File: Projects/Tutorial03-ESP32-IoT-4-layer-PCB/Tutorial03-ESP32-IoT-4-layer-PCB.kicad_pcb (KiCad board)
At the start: 4 copper layers, 149.8 x 55.8 mm, 88 parts, among them J1 SS-52400-002, J2 B2B-PH-SM4-TB, J3 GSD090012SEU, J4 Conn_01x04_Pin, J5 Conn_01x05_Pin, Q1 TEMT6000X01, Q2 BC817, Q3 BC817, U1 MCP73871, U2 MAX4466EXK, U3 ESP32-C3-WROOM-02-H4, U4 CP2102N-Axx-xQFN20, U5 USBLC6-2SC6, U6 W25Q32JVSSIQ, U7 BME280

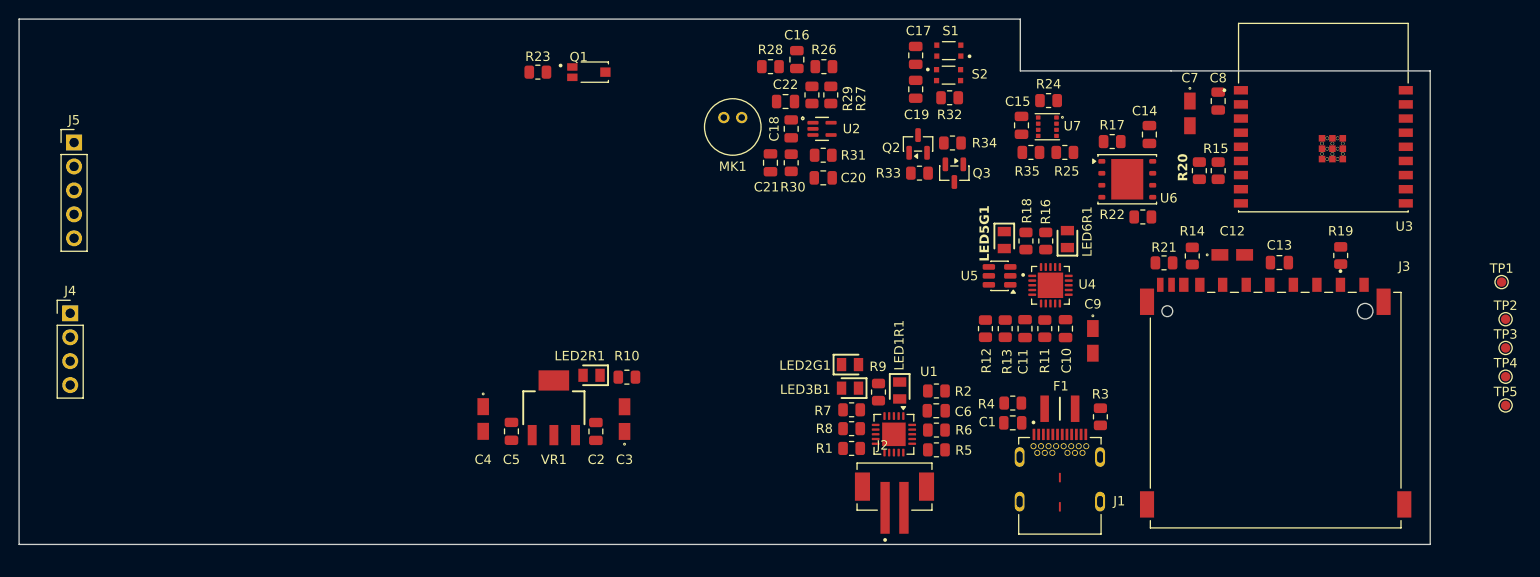
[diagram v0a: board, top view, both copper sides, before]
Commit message: 20260626
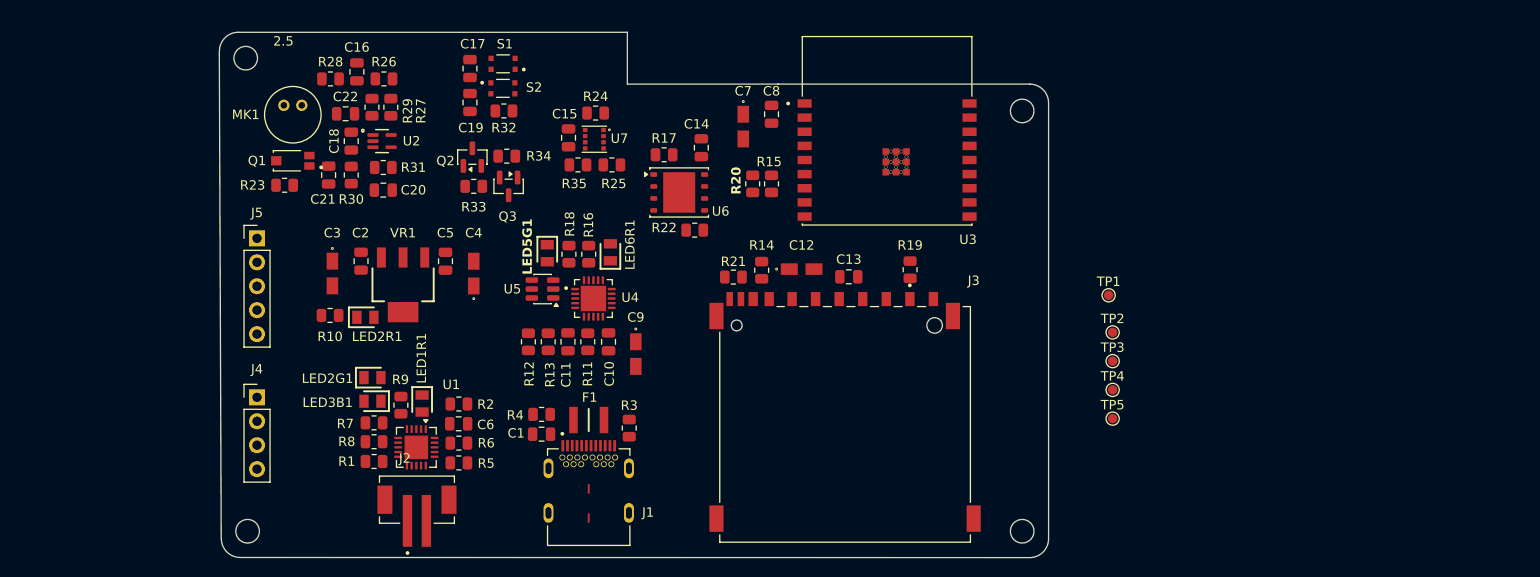
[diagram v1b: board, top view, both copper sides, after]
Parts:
- added 2.5: MountingHole_2.5mm, MountingHole:MountingHole_2.5mm, F.Cu at (179.2, 71.0)
- added 2.5: MountingHole_2.5mm, MountingHole:MountingHole_2.5mm, F.Cu at (179.2, 115.6)
- added 2.5: MountingHole_2.5mm, MountingHole:MountingHole_2.5mm, F.Cu at (96.8, 65.4)
- added REF**: MountingHole_2.5mm, MountingHole:MountingHole_2.5mm, F.Cu at (97.0, 115.6)
- moved C6 50.7 mm to (119.4, 104.2)
- moved J2 50.7 mm to (115.0, 112.2)
- moved LED2G1 50.7 mm to (110.2, 99.3)
- moved LED3B1 50.7 mm to (110.2, 101.8)
- moved U1 50.7 mm to (114.9, 106.7)
- moved LED1R1 50.7 mm to (115.5, 102.0)
- moved R1 50.7 mm to (110.4, 108.2)
- moved R2 50.7 mm to (119.4, 102.1)
- moved R5 50.7 mm to (119.4, 108.3)
- moved R6 50.7 mm to (119.4, 106.2)
- moved R7 50.7 mm to (110.4, 104.1)
- moved R8 50.7 mm to (110.4, 106.1)
- moved R9 50.7 mm to (113.3, 102.2)
- moved C1 50.0 mm to (128.2, 105.3)
- moved F1 50.0 mm to (133.2, 103.8)
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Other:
- board size 149.8 x 55.8 mm -> 88 x 55.8 mm

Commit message: 20260626
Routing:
- added copper zone on In2.Cu, net GND
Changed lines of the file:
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@@
 		(layer "Edge.Cuts")
+	)
+	(zone
+		(net 1)
+		(net_name "GND")
+		(layer "In2.Cu")
+		(name "GND")
+		(hatch edge 0.5)
+		(connect_pads
+			(clearance 0.5)
+		)
+		(min_thickness 0.25)
+		(filled_areas_thickness no)
+		(fill
+			(thermal_gap 0.5)
+			(thermal_bridge_width 0.5)
+		)
+		(polygon
+			(pts
+				(xy 86.8 60.2) (xy 86.8 120.2) (xy 186.2 120.2) (xy 186.6 60.2)
+			)
+		)
 	)
 	(group ""
